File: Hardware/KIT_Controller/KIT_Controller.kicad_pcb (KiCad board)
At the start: 2 copper layers, 1 part, among them U1 LCD

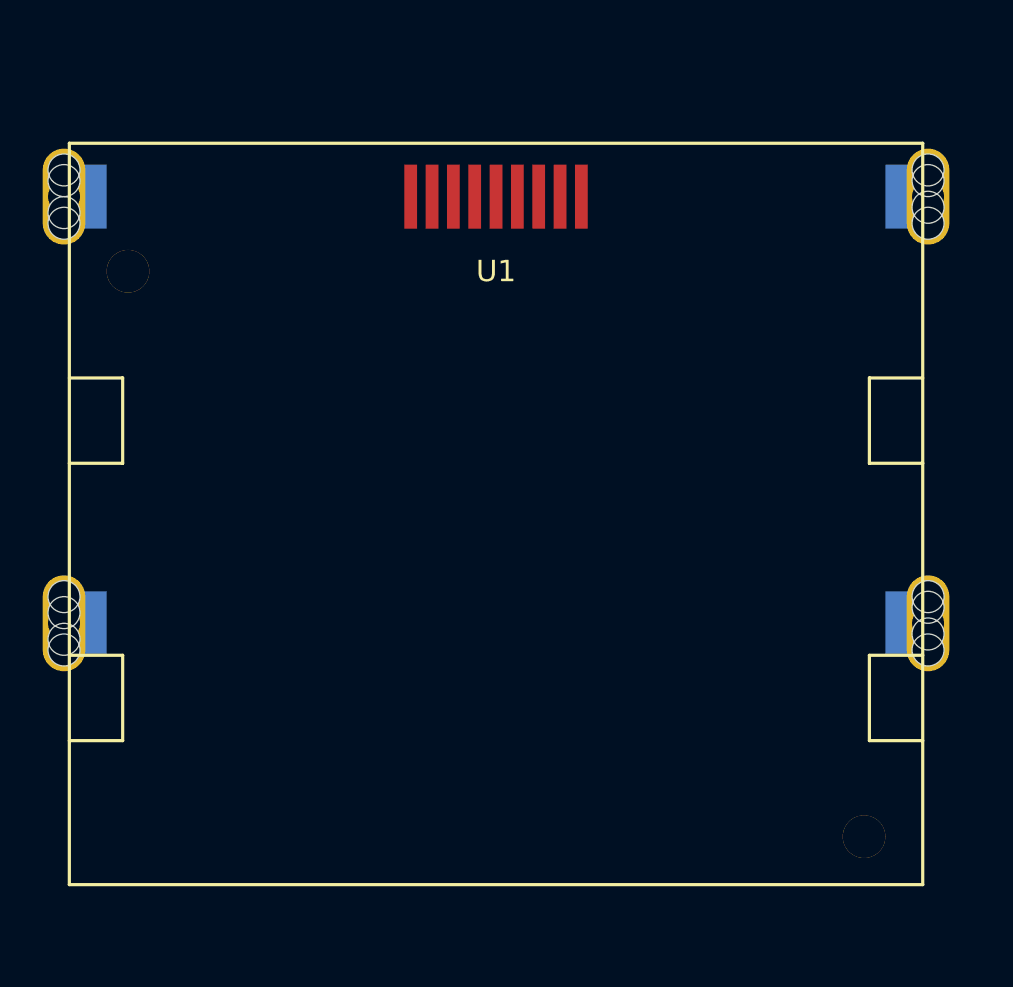
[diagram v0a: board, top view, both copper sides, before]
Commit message: Satisfy constraints
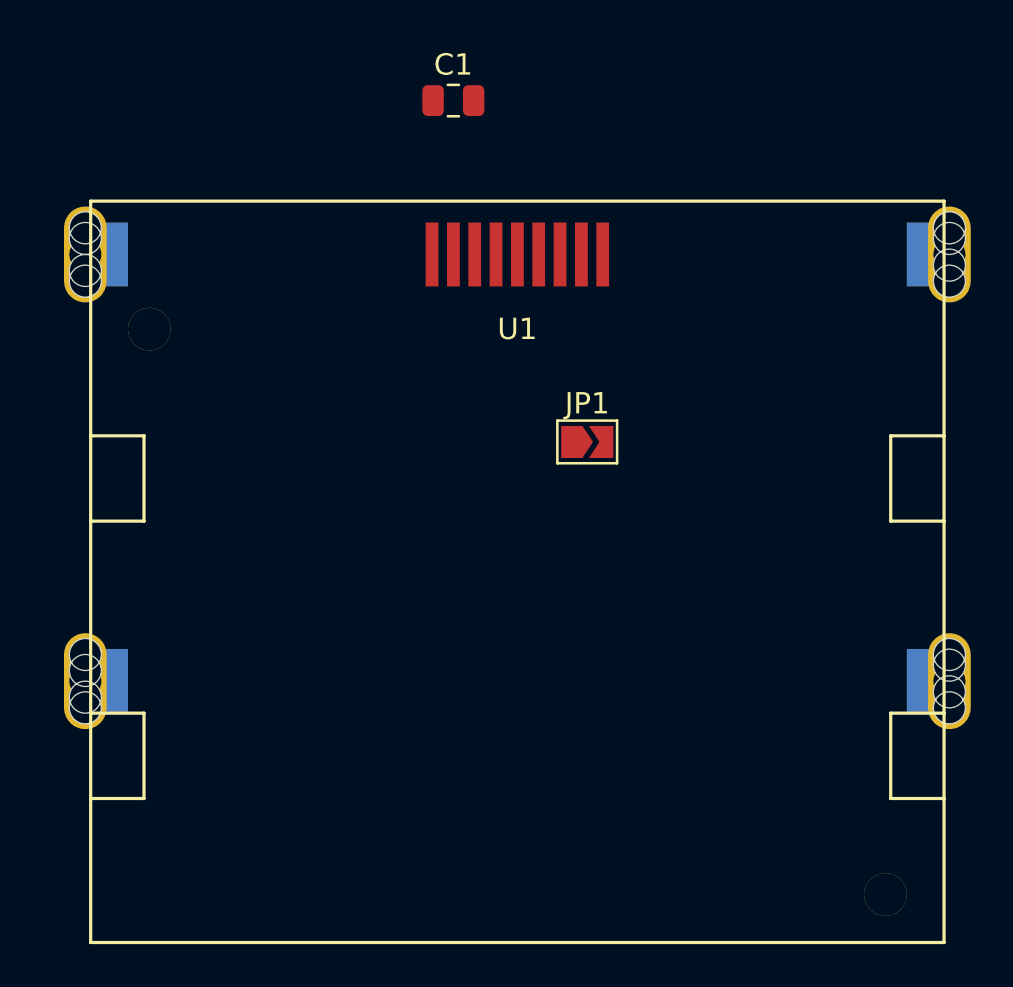
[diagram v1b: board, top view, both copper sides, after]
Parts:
- added C1: 4.7uf, Capacitor_SMD:C_0805_2012Metric, F.Cu at (143.0, 83.0)
- added JP1: SolderJumper_2_Open, Jumper:SolderJumper-2_P1.3mm_Open_TrianglePad1.0x1.5mm, F.Cu at (149.3, 99.0)
- U1: value LCD -> Nokia_5110_LCD
- moved U1 2.89 mm to (146.0, 87.7)
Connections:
- U1 pad 2: unconnected-(U1-Pad2) -> Net-(C1-Pad1)
- U1 pad 3: unconnected-(U1-Pad3) -> GND
- U1 pad 4: unconnected-(U1-Pad4) -> Net-(JP1-Pad1)
- U1 pad 9: unconnected-(U1-Pad9) -> +3.3V
